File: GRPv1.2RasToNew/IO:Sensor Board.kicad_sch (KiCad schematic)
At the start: 45 parts, among them J1 B3B-XH-A, J2 B3B-XH-A, J3 B6B-XH-A, J4 B2B-XH-A, J5 B3B-XH-A, J6 B3B-XH-A, P1 282837-2, P2 282837-2, P3 282837-2, Q1 DMN3023L-7, Q2 DMN3023L-7, Q3 DMN3023L-7, U1 BMP581, U10 XT30UPB-M, U2 DEVKIT_V1_ESP32-WROOM-32, U3 TPS79333-EP, U4 ICM-20948, U5 TPS79318-EP, U7 LD1117S50CTR, U8 XT30UPB-M, U9 LD1117S50CTR

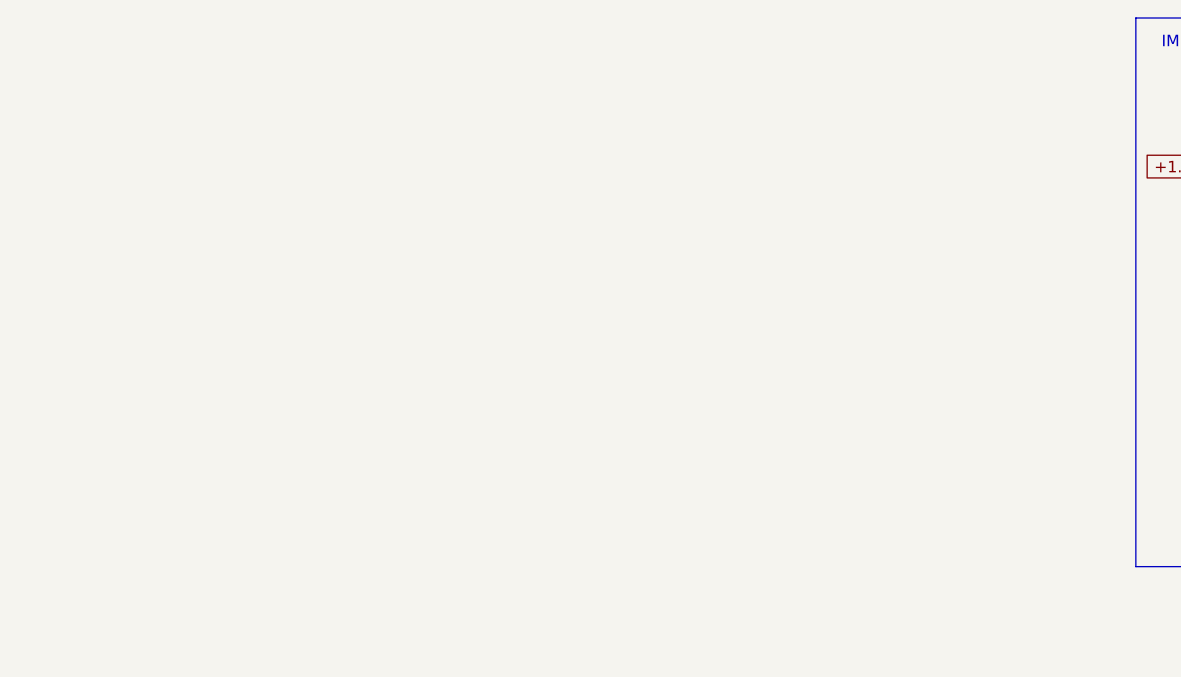
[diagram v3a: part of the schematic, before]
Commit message: oops
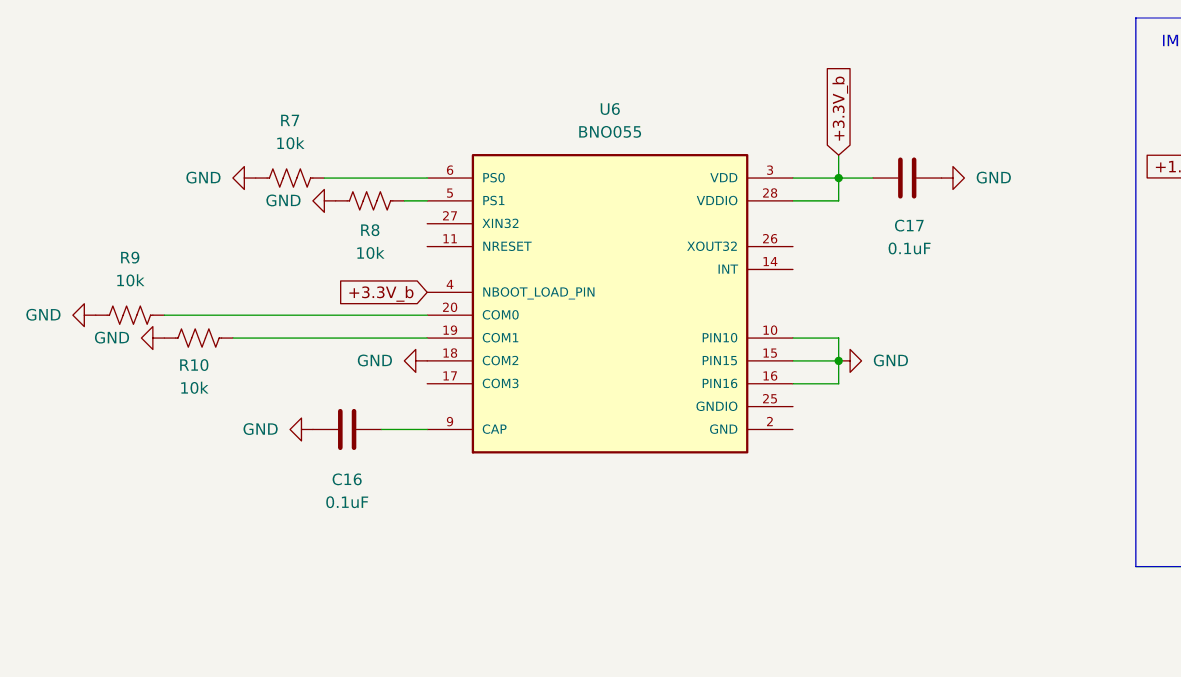
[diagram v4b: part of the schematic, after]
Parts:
- added C16, C17: 0.1uF, Capacitors:C_0805_2012Metric_Pad1.18x1.45mm_HandSolder, symbol Device:C
- added R10, R7, R8, R9: 10k, symbol Device:R_US
- added U6: BNO055, BNO055:LGA28R50P4X10_380X520X100, symbol BNO055:BNO055
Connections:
- net +3.3V_b: now also C17.1, U6.28 (VDDIO), U6.3 (VDD), U6.4 (NBOOT_LOAD_PIN)
- net GND: now also C16.2, C17.2, R10.1, R7.1, R8.2, R9.1, U6.10 (PIN10), U6.15 (PIN15), U6.16 (PIN16), U6.18 (COM2)
- new net: R8.1, U6.5 (PS1)
- new net: R9.2, U6.20 (COM0)
- new net: R7.2, U6.6 (PS0)
- new net: R10.2, U6.19 (COM1)
- new net: C16.1, U6.9 (CAP)
